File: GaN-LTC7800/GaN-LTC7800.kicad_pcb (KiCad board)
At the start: 2 copper layers, 40 parts, among them Q1 EPC2014C, Q2 EPC2014C, U1 LTC7800HUDC_PBF

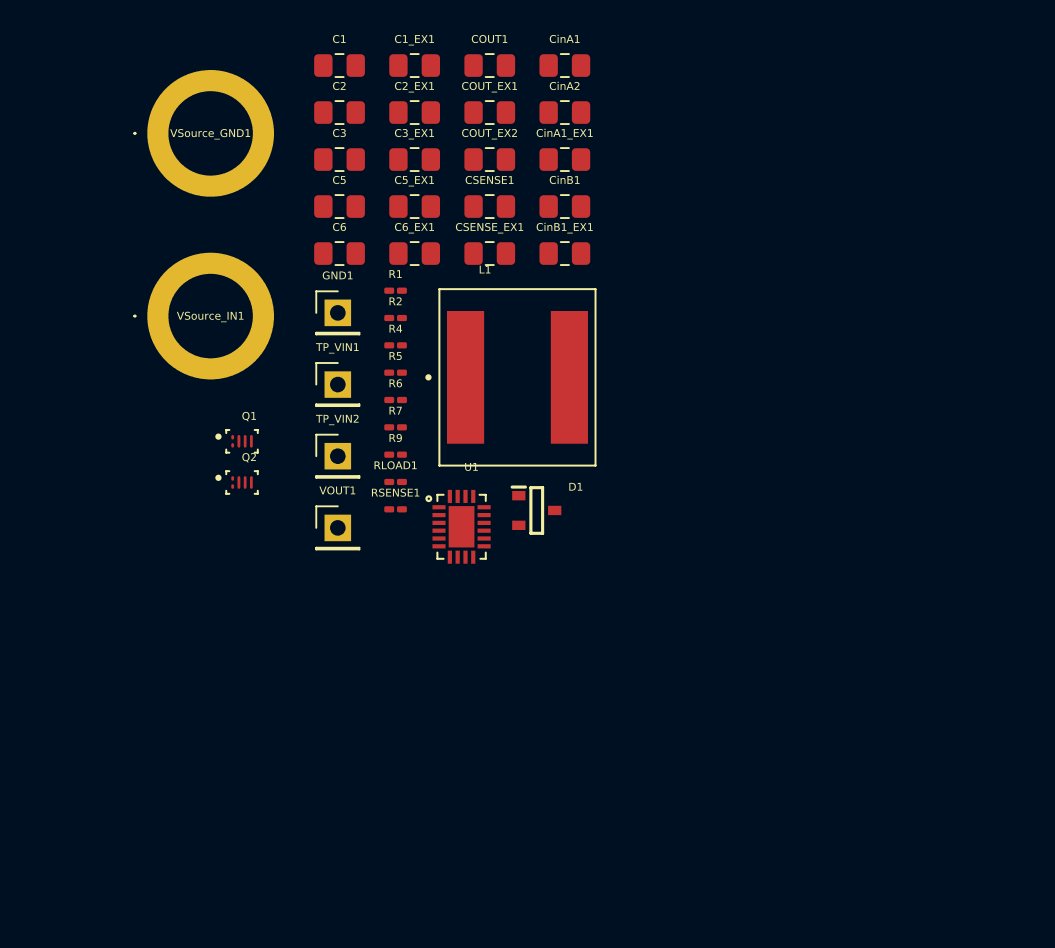
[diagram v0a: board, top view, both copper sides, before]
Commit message: GaN simple layout done
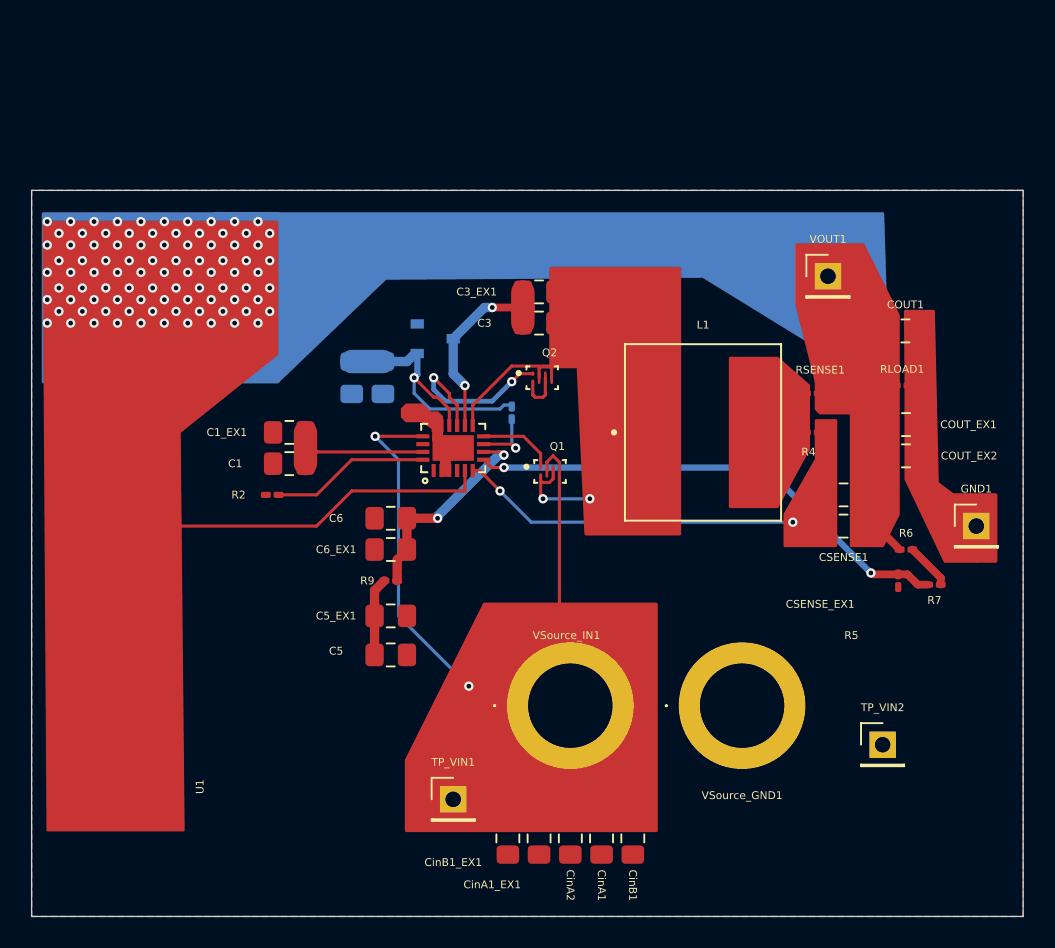
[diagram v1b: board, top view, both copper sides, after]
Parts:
- C2, C2_EX1, D1, R1: moved to B.Cu
- moved VSource_GND1 50.0 mm to (115.0, 150.5)
- moved CinA1 49.6 mm to (106.0, 159.0), turned to -90 degrees
- moved CinA2 46.5 mm to (104.0, 159.0), turned to -90 degrees
- moved CinA1_EX1 43.5 mm to (102.0, 159.0), turned to 90 degrees
- moved GND1 43.1 mm to (130.0, 139.0)
- moved CinB1 40.7 mm to (108.0, 159.0), turned to -90 degrees
- moved TP_VIN2 39.5 mm to (124.0, 153.0)
- moved CinB1_EX1 37.6 mm to (100.0, 159.0), turned to -90 degrees
- moved R7 35.9 mm to (127.3, 142.8), turned to 180 degrees
- moved VOUT1 35.3 mm to (120.5, 123.0)
- moved R5 34.8 mm to (125.0, 142.5), turned to -90 degrees
- moved R6 34.1 mm to (125.5, 140.5)
- moved VSource_IN1 34.0 mm to (104.0, 150.5)
- moved COUT_EX1 33.3 mm to (125.5, 132.5), turned to 180 degrees
- moved RLOAD1 33.0 mm to (125.2, 130.0)
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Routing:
- net /VIN: track 0.00 -> 40.4 mm, vias 0 -> 2
- net /VFB: track 0.00 -> 31.9 mm, vias 0 -> 2
- net /Vout: track 0.00 -> 31.5 mm, vias 0 -> 90
- net /SENSE+: track 0.00 -> 21.9 mm, vias 0 -> 2
- net /SW: track 0.00 -> 19.2 mm, vias 0 -> 2
- net /INTVCC: track 0.00 -> 18.0 mm, vias 0 -> 1
- net /ITH: track 0.00 -> 13.6 mm, vias 0 -> 2
- net /BOOST: track 0.00 -> 13.2 mm, vias 0 -> 2
- net /BG: track 0.00 -> 11.8 mm, vias 0 -> 2
- net Net-(U1-FREQ): track 0.00 -> 10.2 mm
- net Net-(U1-TRACK/SS): track 0.00 -> 9.83 mm
- net GND: track 0.00 -> 5.12 mm
- net Net-(C5-Pad2): track 0.00 -> 5.01 mm
- net /TG: track 0.00 -> 5.00 mm
- net Net-(U1-PGOOD): track 0.00 -> 4.10 mm, vias 0 -> 1
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- added copper zone on B.Cu, net GND
- added copper zone on F.Cu, net GND
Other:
- board outline added: 63.5 x 46.5 mm
